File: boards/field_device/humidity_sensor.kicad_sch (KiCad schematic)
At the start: 3 parts, among them U1 CHT20MEMS

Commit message: assigned better footprints
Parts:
- C1: footprint Capacitor_SMD:C_0603_1608Metric -> Capacitor_SMD:C_0805_2012Metric_Pad1.18x1.45mm_HandSolder
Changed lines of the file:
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@@
 			)
 		)
-		(property "Footprint" "Capacitor_SMD:C_0603_1608Metric"
+		(property "Footprint" "Capacitor_SMD:C_0805_2012Metric_Pad1.18x1.45mm_HandSolder"
 			(at 22.5552 33.02 0)
 			(hide yes)

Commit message: changed regulator
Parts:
- C1: footprint Capacitor_SMD:C_0805_2012Metric_Pad1.18x1.45mm_HandSolder -> Capacitor_SMD:C_0603_1608Metric_Pad1.08x0.95mm_HandSolder
- R1: footprint Resistor_SMD:R_0603_1608Metric -> Resistor_SMD:R_0402_1005Metric_Pad0.72x0.64mm_HandSolder
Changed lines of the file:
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@@
 			)
 		)
-		(property "Footprint" "Resistor_SMD:R_0603_1608Metric"
+		(property "Footprint" "Resistor_SMD:R_0402_1005Metric_Pad0.72x0.64mm_HandSolder"
 			(at 26.67 27.178 90)
 			(hide yes)
@@
 			)
 		)
-		(property "Footprint" "Capacitor_SMD:C_0805_2012Metric_Pad1.18x1.45mm_HandSolder"
+		(property "Footprint" "Capacitor_SMD:C_0603_1608Metric_Pad1.08x0.95mm_HandSolder"
 			(at 22.5552 33.02 0)
 			(hide yes)

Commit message: route more stuff
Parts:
- C1: footprint Capacitor_SMD:C_0603_1608Metric_Pad1.08x0.95mm_HandSolder -> Capacitor_SMD:C_0603_1608Metric
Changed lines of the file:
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@@
 			)
 		)
-		(property "Footprint" "Capacitor_SMD:C_0603_1608Metric_Pad1.08x0.95mm_HandSolder"
+		(property "Footprint" "Capacitor_SMD:C_0603_1608Metric"
 			(at 22.5552 33.02 0)
 			(hide yes)

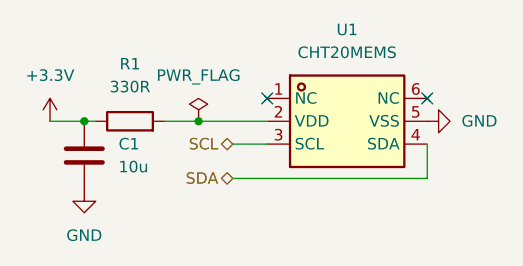
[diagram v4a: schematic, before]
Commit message: rrev 4
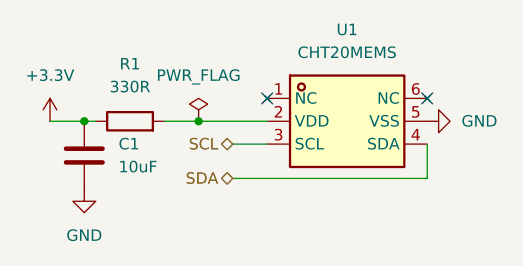
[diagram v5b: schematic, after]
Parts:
- C1: value 10u -> 10uF; footprint Capacitor_SMD:C_0603_1608Metric -> Capacitor_SMD:C_0603_1608Metric_Pad1.08x0.95mm_HandSolder
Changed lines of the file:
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@@
 			)
 		)
-		(property "Value" "10u"
+		(property "Value" "10uF"
 			(at 25.4 30.4799 0)
 			(show_name no)
@@
 			)
 		)
-		(property "Footprint" "Capacitor_SMD:C_0603_1608Metric"
+		(property "Footprint" "Capacitor_SMD:C_0603_1608Metric_Pad1.08x0.95mm_HandSolder"
 			(at 22.5552 33.02 0)
 			(hide yes)

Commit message: Revert "rrev 4"
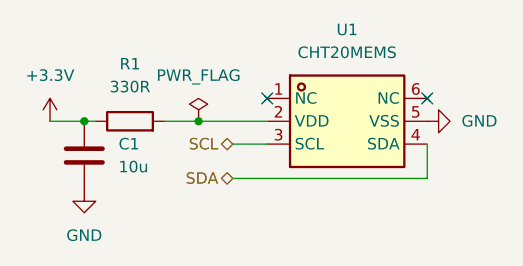
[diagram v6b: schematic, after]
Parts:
- C1: value 10uF -> 10u; footprint Capacitor_SMD:C_0603_1608Metric_Pad1.08x0.95mm_HandSolder -> Capacitor_SMD:C_0603_1608Metric
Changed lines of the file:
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@@
 			)
 		)
-		(property "Value" "10uF"
+		(property "Value" "10u"
 			(at 25.4 30.4799 0)
 			(show_name no)
@@
 			)
 		)
-		(property "Footprint" "Capacitor_SMD:C_0603_1608Metric_Pad1.08x0.95mm_HandSolder"
+		(property "Footprint" "Capacitor_SMD:C_0603_1608Metric"
 			(at 22.5552 33.02 0)
 			(hide yes)
